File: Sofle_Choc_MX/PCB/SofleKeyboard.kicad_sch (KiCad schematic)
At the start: 84 parts, among them J2 4PIN, J3 OLED, P1 i2c_pin, P2 i2c_pin, SW1 SW_PUSH_LED, SW10 SW_PUSH_LED, SW11 SW_PUSH_LED, SW12 SW_PUSH_LED, SW13 SW_PUSH_LED, SW14 SW_PUSH_LED, SW15 SW_PUSH_LED, SW16 SW_PUSH_LED, SW17 SW_PUSH_LED, SW18 SW_PUSH_LED, SW19 SW_PUSH_LED, SW2 SW_PUSH_LED, SW20 SW_PUSH_LED, SW21 SW_PUSH_LED, SW22 SW_PUSH_LED, SW23 SW_PUSH_LED, SW24 SW_PUSH_LED, SW25 Rotary_Encoder_Switch, SW26 SW_PUSH_LED, SW27 SW_PUSH_LED, SW28 SW_PUSH_LED, SW29 SW_PUSH_LED, SW3 SW_PUSH_LED, SW30 SW_PUSH_LED, SW4 SW_PUSH_LED, SW5 SW_PUSH_LED, SW6 SW_PUSH_LED, SW7 SW_PUSH_LED, SW8 SW_PUSH_LED, SW9 SW_PUSH_LED, U1 ProMicro_Choc_MX

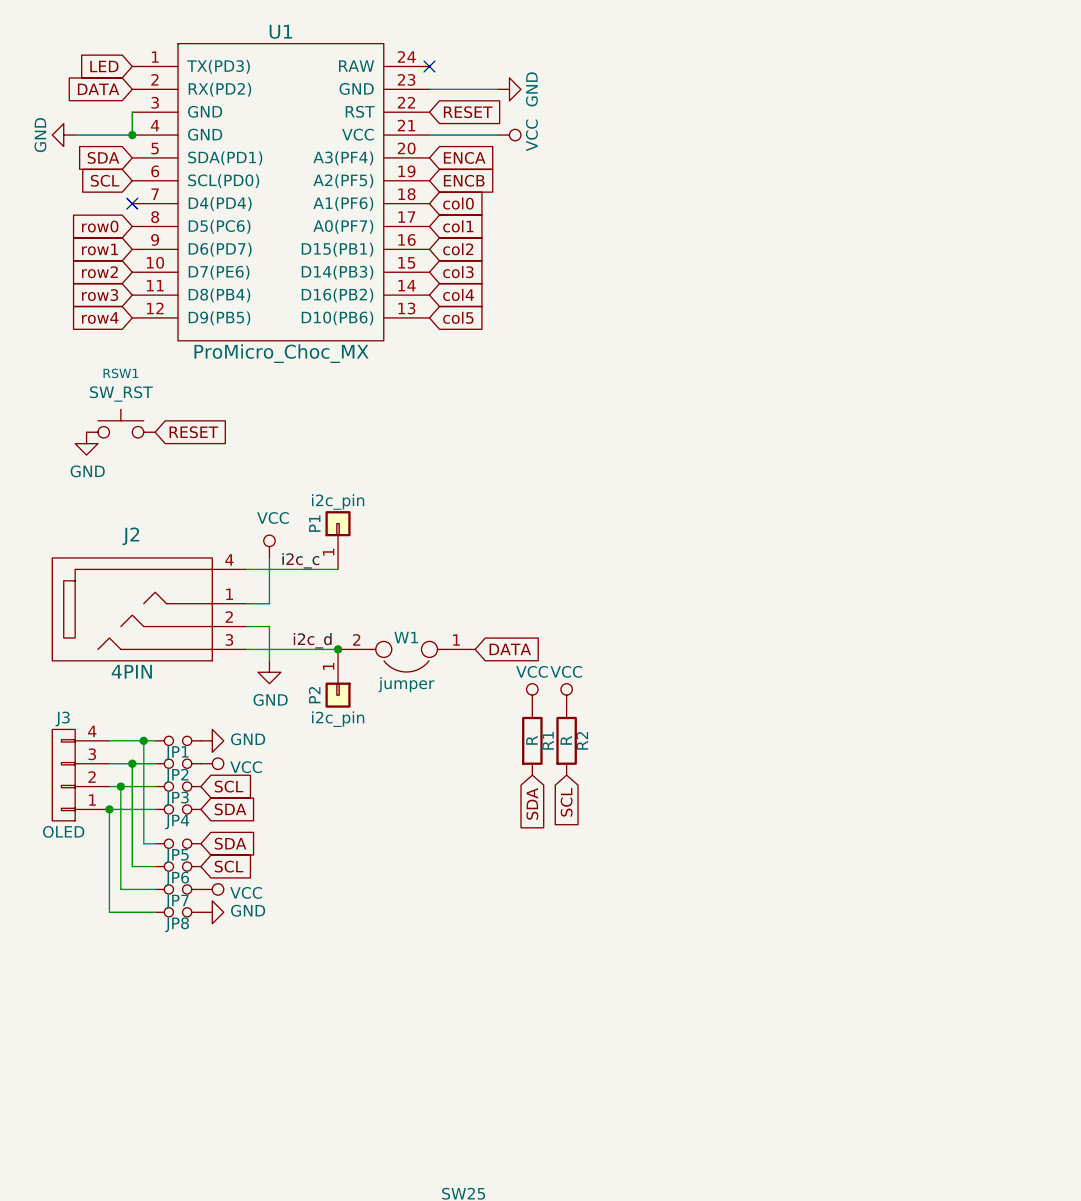
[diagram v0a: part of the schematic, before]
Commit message: Sent this version out for production at jlcpcb
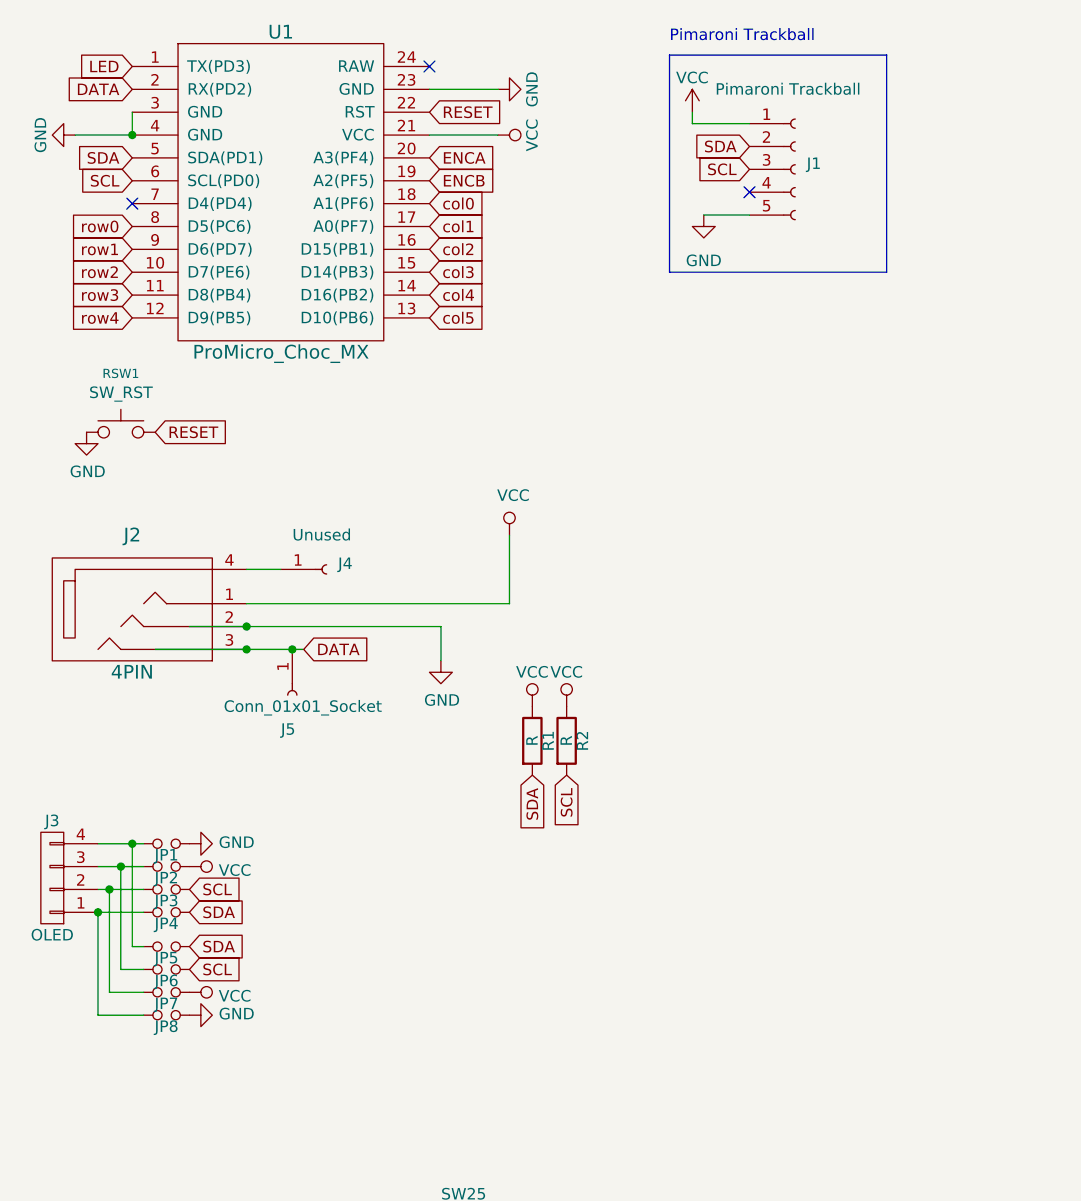
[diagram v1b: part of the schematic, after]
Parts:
- removed P1, P2: i2c_pin, SofleKeyboard-footprint:1pin_conn, symbol SofleKeyboard-rescue:i2c_pin-Lily58-cache-Lily58_Pro-rescue
- removed W1: jumper, SofleKeyboard-footprint:jumper_data, symbol SofleKeyboard-rescue:Jumper-Device
- added J1: Pimaroni Trackball, SofleChoc:Pimaroni_PinHeader_1x05_P2.54mm_Vertical, symbol Connector:Conn_01x05_Socket
- added J4: Unused, SofleChoc:1pin_conn, symbol Connector:Conn_01x01_Socket
- added J5: Conn_01x01_Socket, SofleChoc:1pin_conn, symbol Connector:Conn_01x01_Socket
- J2: footprint SofleKeyboard-footprint:MJ-4PP-9 -> SofleChoc:MJ-4PP-9_Choc_MX
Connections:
- net i2c_d is gone; now on net DATA: J2.3
- net DATA: now also J5.1 (Pin_1)
- net GND: now also J1.5 (Pin_5)
- net SCL: now also J1.3 (Pin_3)
- net SDA: now also J1.2 (Pin_2)
- net VCC: now also J1.1 (Pin_1)
- net i2c_c: no longer names the net of J2.4
- net i2c_c: now also J4.1 (Pin_1)
- no-connect marks 3 -> 4
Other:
- note added: "Pimaroni Trackball"
- moved on the sheet: J3, JP1, JP2, JP3, JP4, JP5, JP6, JP7, JP8
